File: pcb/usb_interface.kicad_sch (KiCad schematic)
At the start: 8 parts, among them J12 USB_C_Receptacle

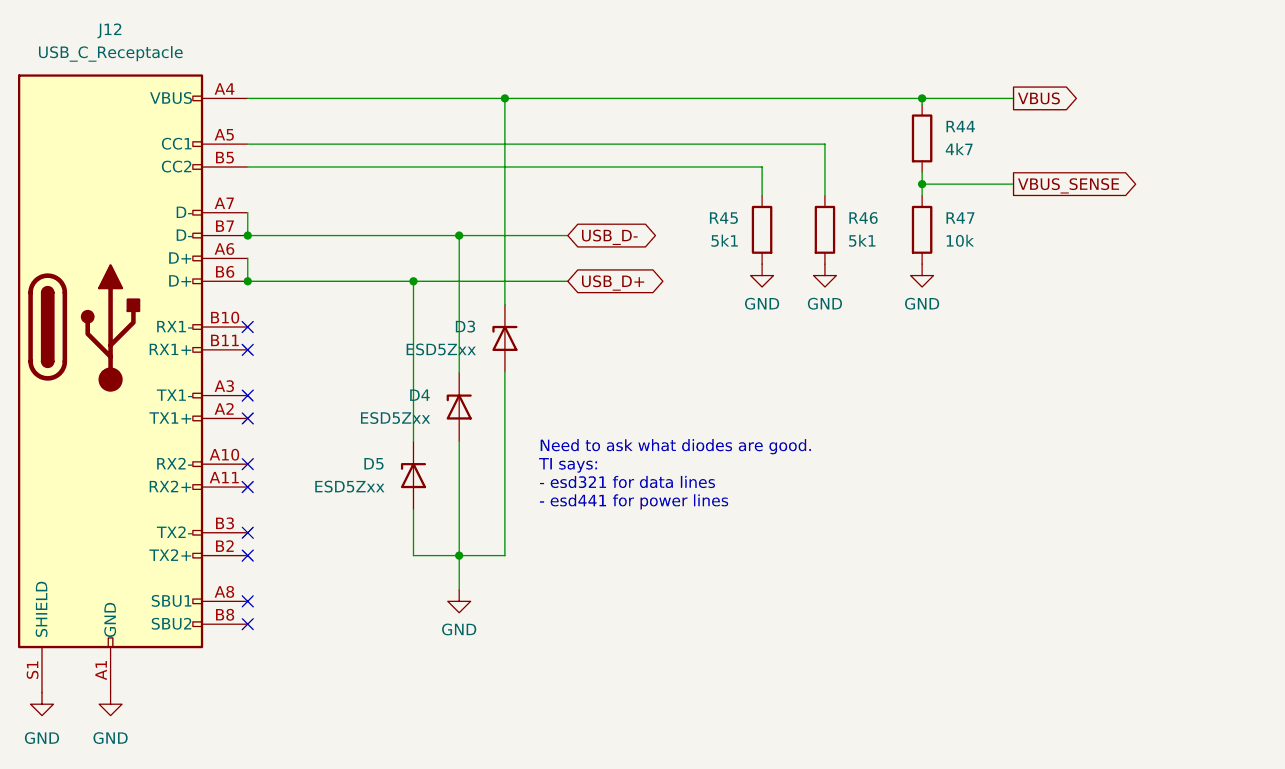
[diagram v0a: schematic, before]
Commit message: starting the revision from ed
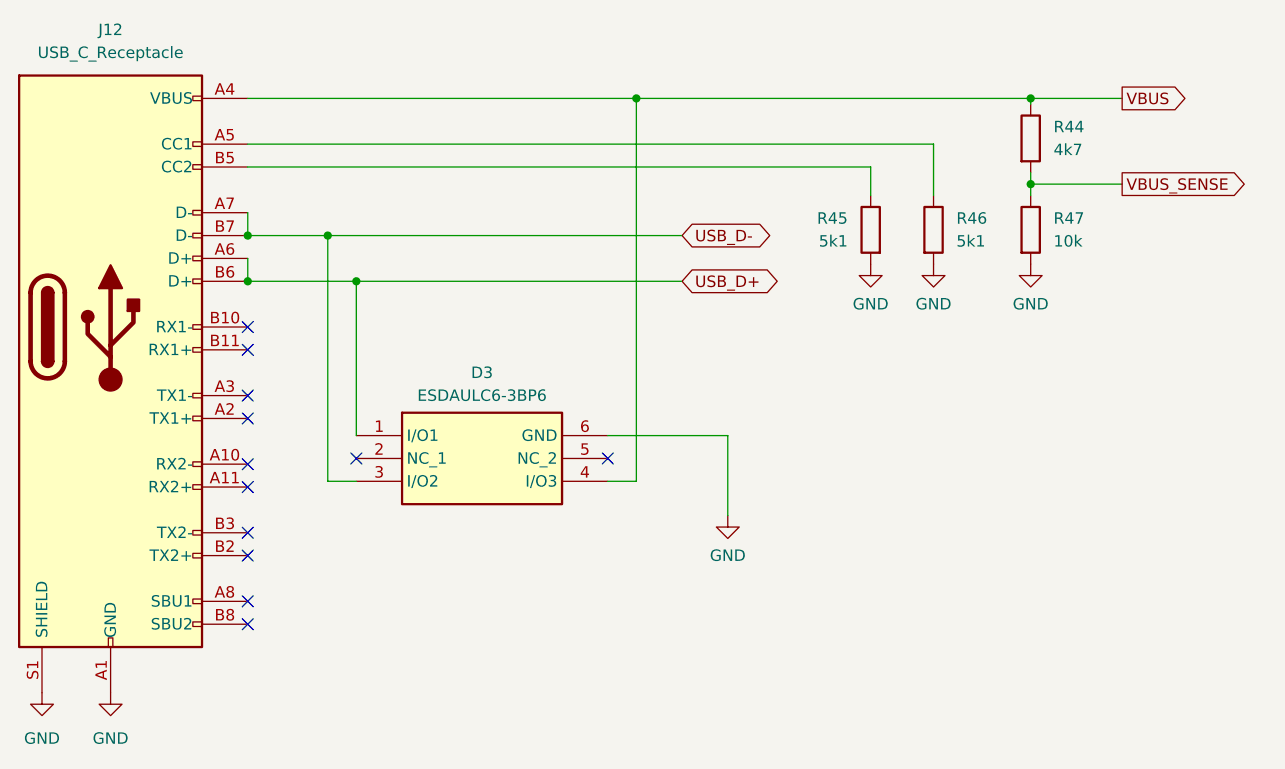
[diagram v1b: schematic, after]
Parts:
- removed D3, D4, D5: ESD5Zxx, Diode_SMD:D_SOD-523, symbol Diode:ESD5Zxx
- added D3: ESDAULC6-3BP6, ESDAULC63BP6, symbol library:ESDAULC6-3BP6
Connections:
- net GND: now also D3.6 (GND)
- net USB_D+: now also D3.1 (I/O1)
- net USB_D-: now also D3.3 (I/O2)
- net VBUS: now also D3.4 (I/O3)
- no-connect marks 10 -> 12
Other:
- note removed: "Need to ask what diodes are good. TI says: - esd321 for data lines - esd441 for power lines"
- moved on the sheet: R44, R45, R46, R47

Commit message: progress
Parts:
- D3: footprint ESDAULC63BP6 -> library:ESDAULC63BP6
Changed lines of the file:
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@@
       (effects (font (size 1.27 1.27)))
     )
-    (property "Footprint" "ESDAULC63BP6" (at 156.845 208.585 0)
+    (property "Footprint" "library:ESDAULC63BP6" (at 156.845 208.585 0)
       (effects (font (size 1.27 1.27)) (justify left top) hide)
     )
@@
     (pin "1")
     (pin "2")
+    (pin "3")
     (pin "4")
     (pin "5")
-    (pin "3")
     (pin "6")
     (instances
